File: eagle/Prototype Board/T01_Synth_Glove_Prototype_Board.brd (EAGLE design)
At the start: 76.2 x 76.2 mm, 61 parts, among them SW1 RESET_BUTTON, U1 ATMEGA328P, U2 ZLDO1117

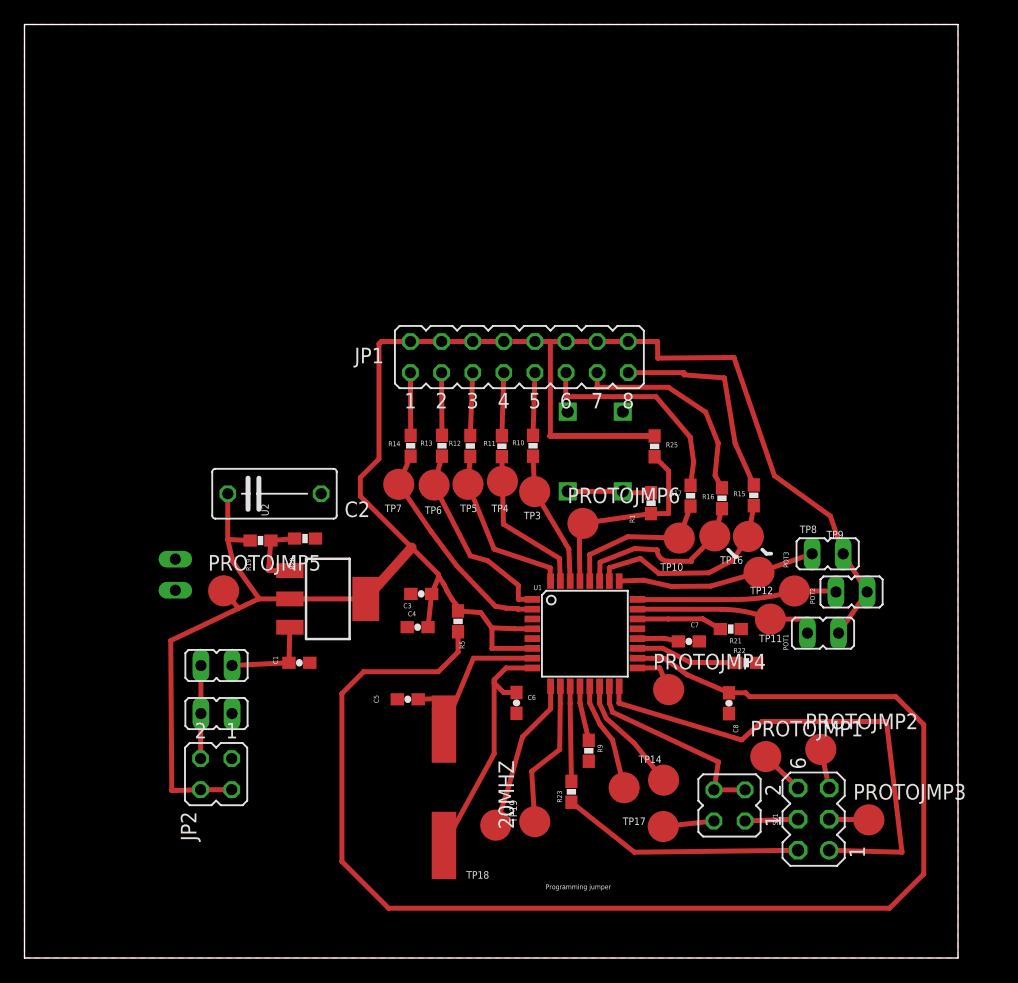
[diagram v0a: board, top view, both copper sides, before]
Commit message: Update, more CAM files
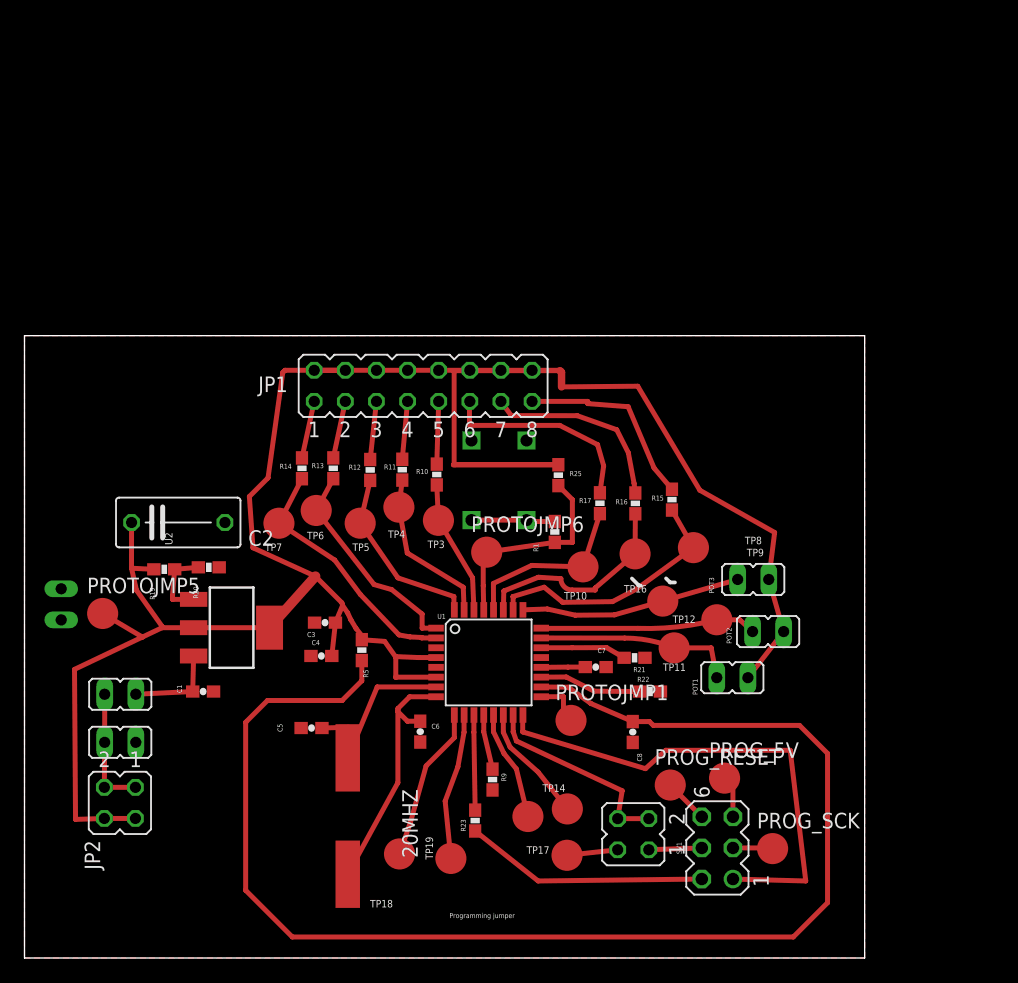
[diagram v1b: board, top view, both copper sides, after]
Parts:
- removed PROTOJMP2, PROTOJMP3, PROTOJMP4: PTR1B2,54, testpad:B2,54
- added PROG_5V, PROG_RESET, PROG_SCK: PTR1B2,54, testpad:B2,54
- moved PROTOJMP1 16.2 mm to (44.6, 19.4)
- moved TP7 10.3 mm to (20.8, 35.5)
- moved PROTOJMP5 10.0 mm to (6.38, 28.1)
- moved TP6 9.84 mm to (23.8, 36.5)
- moved JP3 9.62 mm to (3.00, 28.9)
- moved TP5 9.35 mm to (27.4, 35.5)
- moved R13 9.06 mm to (25.2, 40.0)
- moved R14 9.06 mm to (22.6, 40.0)
- moved TP4 8.71 mm to (30.6, 36.8)
- moved R12 8.40 mm to (28.2, 39.8)
- moved R11 8.35 mm to (30.8, 39.9)
- moved POT1 8.25 mm to (57.8, 22.9)
- moved C8 8.20 mm to (49.7, 18.4)
- moved C3 8.20 mm to (24.5, 27.4)
- moved C1 8.20 mm to (14.6, 21.8)
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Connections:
- new net JP3: PROG_SCK.TP, SV1.3
- new net N$2: PROG_5V.TP, SV1.5
- new net PJ4: PROG_RESET.TP, SV1.6
- net +5V: no longer PROTOJMP2.TP, SV1.5
- net RESET: no longer PROTOJMP3.TP, SV1.3
- net SCK: no longer PROTOJMP4.TP, SV1.6
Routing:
- net +5V: track 182.0 -> 195.3 mm
- net PC3: track 16.8 -> 21.3 mm
- net PJ4: track 0.00 -> 3.66 mm
- net N$2: track 0.00 -> 3.44 mm
- net SCK: track 7.41 -> 4.00 mm
- net JP3: track 0.00 -> 3.26 mm
- net RESET: track 20.4 -> 17.2 mm
- net PC4: track 14.8 -> 17.3 mm
- net +9V: track 7.60 -> 10.1 mm
- net PD4: track 18.3 -> 20.7 mm
- net PC5: track 12.6 -> 14.4 mm
- net PC2: track 16.2 -> 18.0 mm
- net PD3: track 15.9 -> 17.6 mm
- net N$15: track 17.2 -> 15.7 mm
- net N$13: track 17.2 -> 15.7 mm
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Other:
- board size 76.2 x 76.2 mm -> 68.6 x 50.8 mm
